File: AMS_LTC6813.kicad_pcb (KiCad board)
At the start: 2 copper layers, 204 parts, among them J1 Conn_01x06, J10 Conn_01x02_Male, J11 Conn_01x02_Male, J12 Conn_01x02_Male, J13 Conn_01x02_Male, J14 Conn_01x02_Male, J15 Conn_01x02_Male, J16 Conn_01x02_Male, J17 Conn_01x02_Male, J18 Conn_01x02_Male, J19 Conn_01x02_Male, J20 Conn_01x02_Male, J21 Conn_01x02_Male, J22 Conn_01x02_Male, J23 Conn_01x02_Male, J24 Conn_01x02_Male, J25 Conn_01x02_Male, J26 Conn_01x02_Male, J27 Conn_01x02_Male, J28 Conn_01x02_Male, J29 Conn_01x02_Male, J3 Conn_01x06, J30 Conn_01x02_Male, J31 Conn_01x02_Male, J32 Conn_01x02_Male, J33 Conn_01x02_Male, J34 Conn_01x02_Male, J35 Conn_01x02_Male, J36 Conn_01x02_Male, J37 Conn_01x02_Male, J38 Conn_01x02_Male, J39 Conn_01x02_Male, J4 Conn_02x02_Counter_Clockwise, J40 Conn_01x02_Male, J41 Conn_01x02_Male, J42 Conn_01x02_Male, J43 Conn_01x02_Male, J44 Conn_01x02_Male, J45 Conn_01x02_Male, J46 Conn_01x02_Male, J47 Conn_01x02_Male, J48 Conn_01x02_Male, J49 Conn_01x02_Male, J5 Conn_01x02_Male, J50 Conn_01x02_Male, J51 Conn_01x02_Male, J52 Conn_01x02_Male, J53 Conn_01x02_Male, J54 Conn_01x02_Male, J55 Conn_01x02_Male, J56 Conn_01x02_Male, J57 Conn_01x02_Male, J58 Conn_01x02_Male, J59 Conn_01x02_Male, J6 Conn_01x02_Male, J60 Conn_01x02_Male, J61 Conn_01x02_Male, J62 Conn_01x02_Male, J63 Conn_01x02_Male, J64 Conn_01x02_Male, J65 Conn_01x02_Male, J66 Conn_01x02_Male, J67 Conn_01x02_Male, J68 Conn_01x02_Male, J69 Conn_02x02_Counter_Clockwise, J7 Conn_01x02_Male, J70 Conn_01x03_Female, J71 Conn_02x20_Counter_Clockwise, J72 Conn_01x02_Male, J73 Conn_01x02_Male, J74 Conn_01x02_Male, J75 Conn_01x02_Male, J76 Conn_01x02_Male, J77 Conn_01x02_Male, J78 Conn_01x02_Male, J79 Conn_01x02_Male, J8 Conn_01x02_Male, J80 Conn_01x02_Male, J81 Conn_01x02_Male, J82 Conn_01x02_Male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

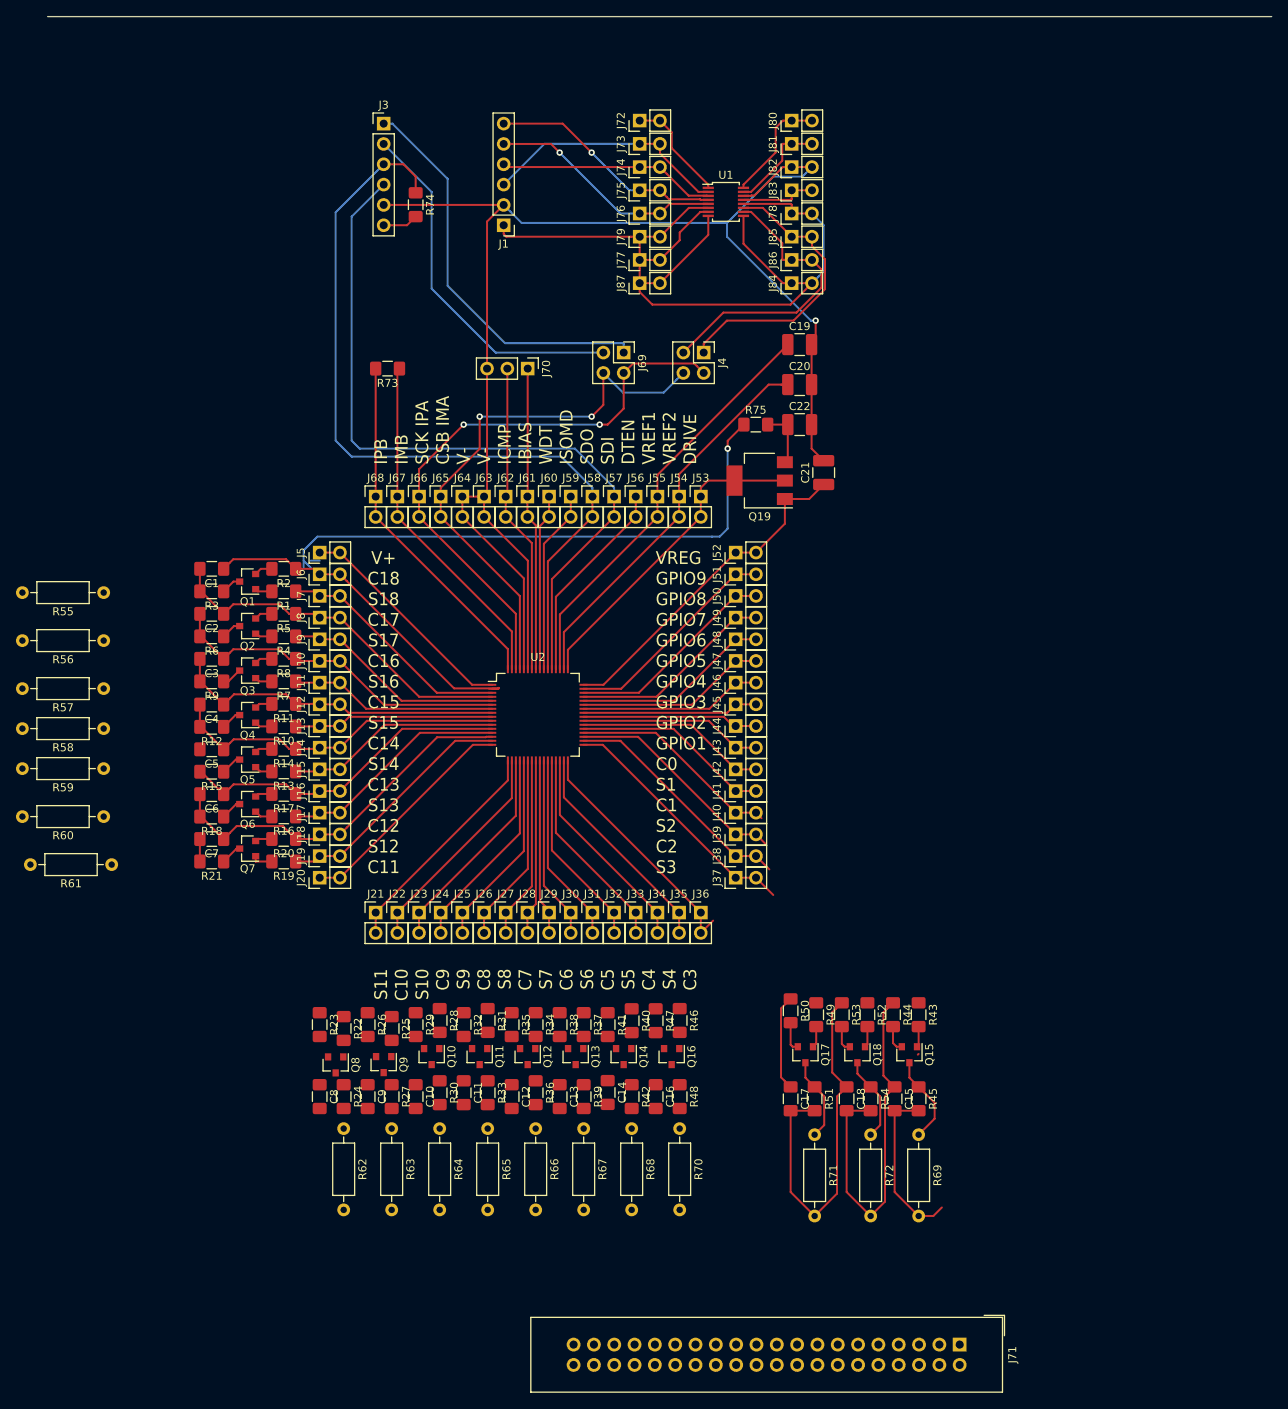
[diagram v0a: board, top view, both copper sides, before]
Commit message: routing everything
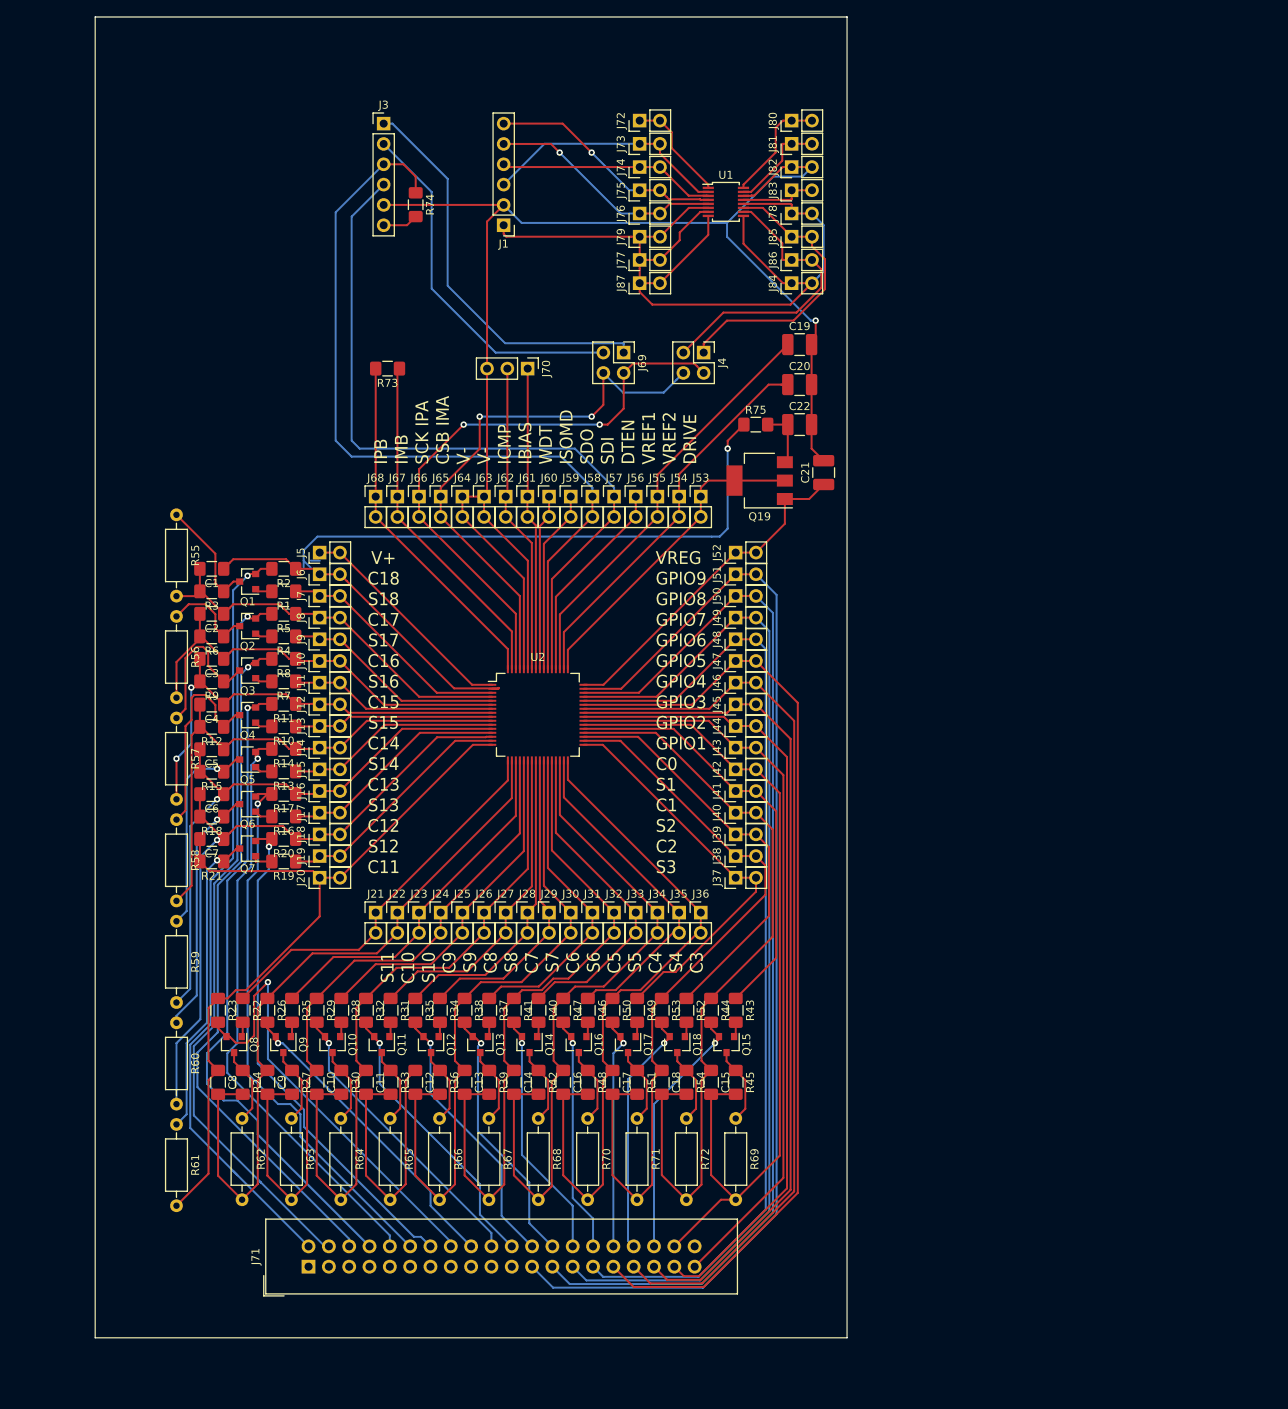
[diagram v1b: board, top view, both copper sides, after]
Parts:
- moved J71 82.0 mm to (54.6, 175.3), turned to 90 degrees
- moved R61 33.5 mm to (38.1, 157.5), turned to 270 degrees
- moved R60 27.3 mm to (38.1, 144.8), turned to 270 degrees
- moved C18 23.2 mm to (98.8, 152.2)
- moved R72 23.1 mm to (101.8, 156.7)
- moved R54 23.1 mm to (101.8, 152.2)
- moved C15 23.0 mm to (104.9, 152.2)
- moved R45 23.0 mm to (108.0, 152.2)
- moved R69 23.0 mm to (108.0, 156.7)
- moved Q15 22.9 mm to (106.9, 147.5)
- moved R43 22.9 mm to (108.0, 143.2)
- moved R44 22.7 mm to (104.9, 143.2)
- moved R52 22.6 mm to (101.8, 143.2)
- moved Q18 22.6 mm to (100.7, 147.5)
- moved R53 22.5 mm to (98.8, 143.2)
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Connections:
- J71 pad 10: /CELL10 -> /CELL14
- J71 pad 11: /CELL9 -> Net-(J71-Pad11)
- J71 pad 12: /CELL8 -> /CELL13
- J71 pad 13: /CELL7 -> Net-(J71-Pad13)
- J71 pad 14: /CELL6 -> /CELL12
- J71 pad 15: /CELL5 -> Net-(J71-Pad15)
- J71 pad 16: /CELL4 -> /CELL11
- J71 pad 17: /CELL3 -> Net-(J71-Pad17)
- J71 pad 18: /CELL2 -> /CELL10
- J71 pad 19: /CELL1 -> Net-(J71-Pad19)
- J71 pad 20: /C0 -> /CELL9
- J71 pad 21: /GPIO1 -> Net-(J71-Pad21)
- J71 pad 22: /GPIO2 -> /CELL8
- J71 pad 23: /GPIO3 -> /GPIO9
- J71 pad 24: /GPIO4 -> /CELL7
- J71 pad 25: /GPIO5 -> /GPIO8
- J71 pad 26: /GPIO6 -> /CELL6
- J71 pad 28: /GPIO8 -> /CELL5
- J71 pad 29: /GPIO9 -> /GPIO6
- J71 pad 3: /CELL17 -> Net-(J71-Pad3)
- J71 pad 30: Net-(J71-Pad30) -> /CELL4
- J71 pad 31: Net-(J71-Pad31) -> /GPIO5
- J71 pad 32: Net-(J71-Pad32) -> /CELL3
- J71 pad 33: Net-(J71-Pad33) -> /GPIO4
- J71 pad 34: Net-(J71-Pad34) -> /CELL2
- J71 pad 35: Net-(J71-Pad35) -> /GPIO3
- J71 pad 36: Net-(J71-Pad36) -> /CELL1
- J71 pad 37: Net-(J71-Pad37) -> /GPIO2
- J71 pad 38: Net-(J71-Pad38) -> /C0
- J71 pad 39: Net-(J71-Pad39) -> /GPIO1
- J71 pad 4: /CELL16 -> /CELL17
- J71 pad 5: /CELL15 -> Net-(J71-Pad5)
- J71 pad 6: /CELL14 -> /CELL16
- J71 pad 7: /CELL13 -> Net-(J71-Pad7)
- J71 pad 8: /CELL12 -> /CELL15
- J71 pad 9: /CELL11 -> Net-(J71-Pad9)
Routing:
- net /GPIO9: track 27.5 -> 144.0 mm
- net /GPIO8: track 26.6 -> 136.7 mm
- net /GPIO7: track 25.7 -> 129.4 mm
- net /GPIO5: track 23.8 -> 121.5 mm
- net /GPIO6: track 24.7 -> 122.1 mm
- net /CELL18: track 2.29 -> 97.1 mm, vias 0 -> 1
- net /GPIO4: track 22.9 -> 114.2 mm
- net /CELL17: track 2.26 -> 92.7 mm, vias 0 -> 1
- net /GPIO3: track 22.0 -> 106.9 mm
- net /CELL16: track 2.24 -> 86.3 mm, vias 0 -> 1
- net /CELL15: track 2.21 -> 82.1 mm, vias 0 -> 1
- net /GPIO2: track 22.0 -> 100.6 mm
- net /CELL14: track 2.18 -> 74.1 mm, vias 0 -> 1
- net /GPIO1: track 23.0 -> 93.8 mm
- net /CELL13: track 2.16 -> 69.6 mm, vias 0 -> 1
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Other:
- board outline added: 94 x 165.2 mm
